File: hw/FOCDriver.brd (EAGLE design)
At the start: 99.1 x 68 mm, 106 parts, among them U1 IX4428N, U2 IX4428N, U3 IX4428N, U4 IRF9389TRPBF, U5 IRF9389TRPBF, U6 IRF9389TRPBF, U7 LM27313XMF, U8 MCP6024T-I, U9 TLV3201AIDBVR

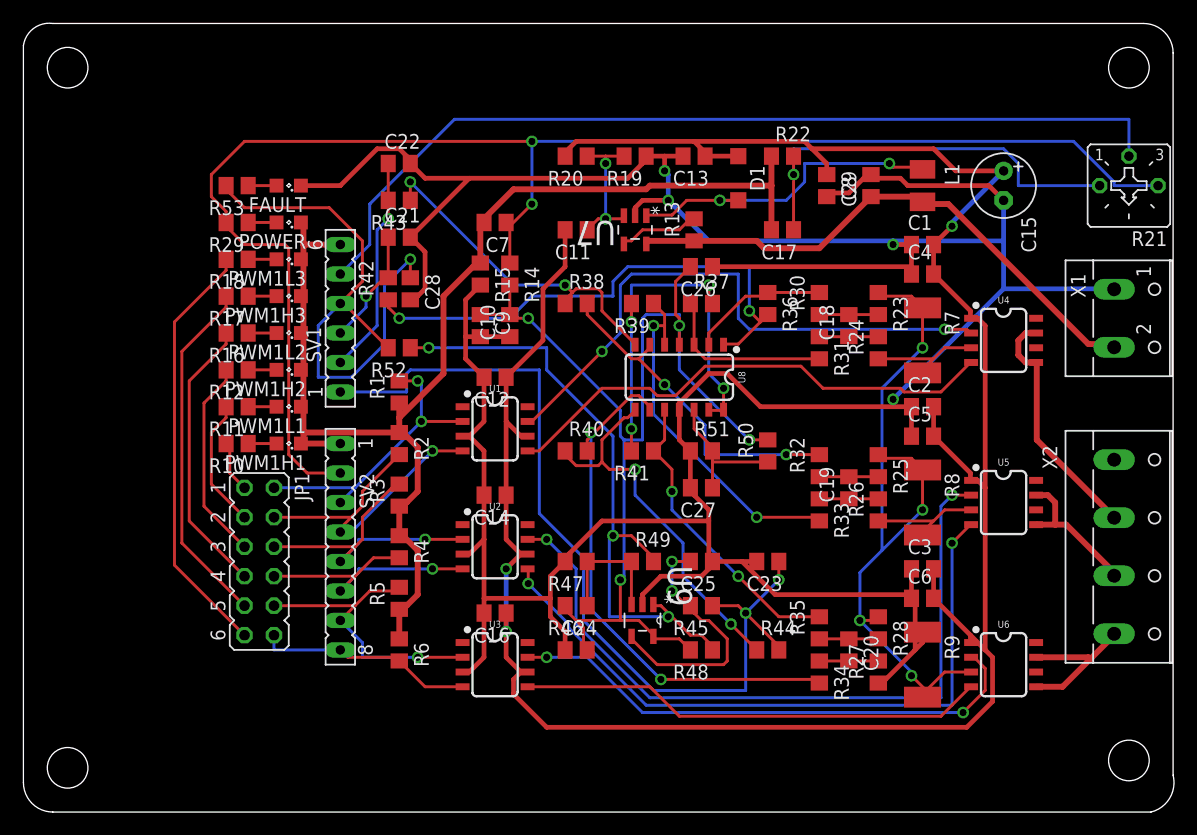
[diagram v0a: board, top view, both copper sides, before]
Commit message: layout
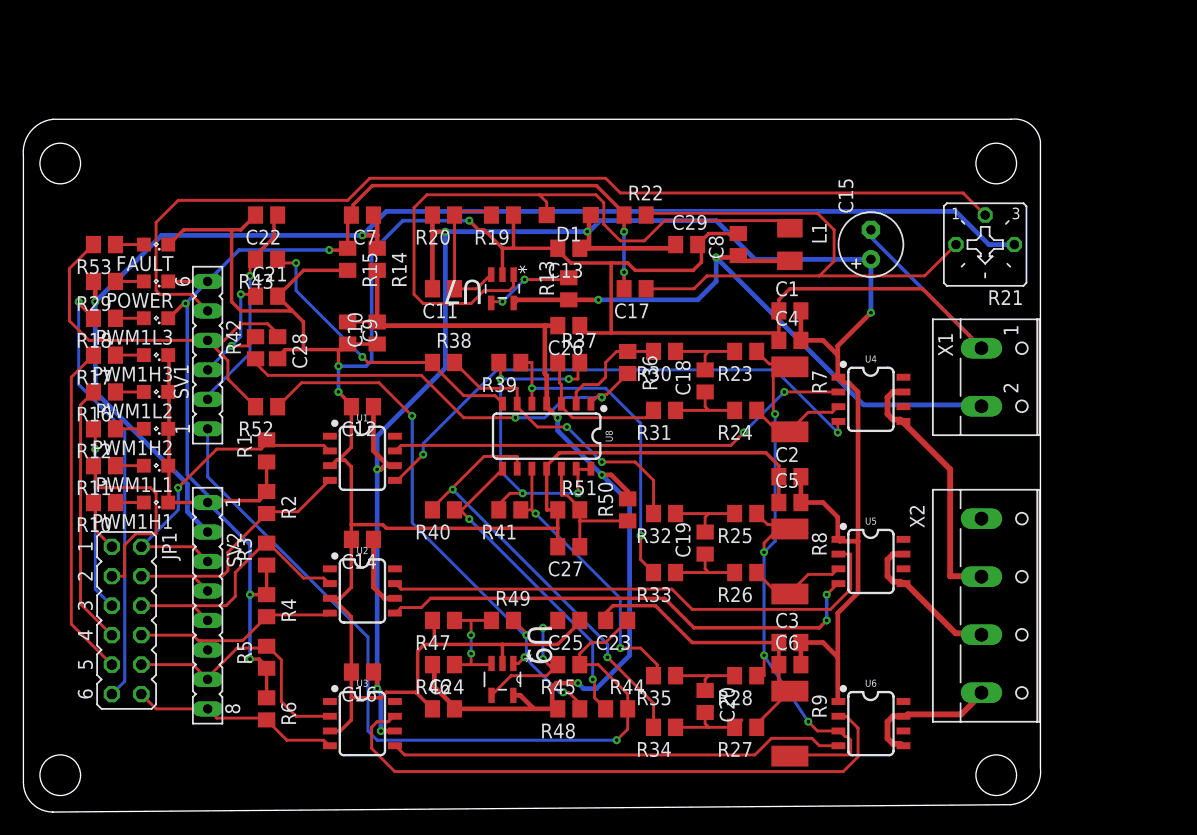
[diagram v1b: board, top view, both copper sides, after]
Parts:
- moved D1 14.9 mm to (47.0, 51.4), turned to 180 degrees
- moved R31 14.4 mm to (55.2, 34.6), turned to 180 degrees
- moved R33 14.4 mm to (55.2, 20.6), turned to 180 degrees
- moved R34 14.2 mm to (55.2, 7.30), turned to 180 degrees
- moved C23 14.0 mm to (51.1, 16.5)
- moved R44 14.0 mm to (51.1, 8.89)
- moved R30 14.0 mm to (55.2, 39.7), turned to 180 degrees
- moved R32 14.0 mm to (55.2, 25.7), turned to 180 degrees
- moved R35 14.0 mm to (55.2, 11.7), turned to 180 degrees
- moved C17 13.7 mm to (52.7, 45.1)
- moved R22 13.7 mm to (52.7, 51.4)
- moved C13 13.4 mm to (47.0, 48.6)
- moved R21 13.4 mm to (82.9, 48.9)
- moved C19 13.3 mm to (58.7, 23.2)
- moved C18 13.3 mm to (58.7, 37.1)
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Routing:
- net N$5: track 28.5 -> 56.6 mm, vias 2 -> 0
- net +12V: track 210.5 -> 183.3 mm, vias 3 -> 6
- net N$8: track 63.6 -> 45.0 mm, vias 2 -> 0
- net +3V3: track 130.9 -> 113.8 mm
- net N$7: track 58.6 -> 42.7 mm
- net FAULT_MC: track 49.8 -> 35.2 mm, vias 1 -> 0
- net N$29: track 37.4 -> 49.6 mm, vias 1 -> 0
- net N$27: track 23.7 -> 12.7 mm
- net N$10: track 50.2 -> 40.3 mm
- net IMOTORBUS: track 78.5 -> 69.3 mm, vias 2 -> 1
- net N$16: track 46.1 -> 37.5 mm
- net AGND: track 314.6 -> 306.0 mm, vias 4 -> 3
- net GND: track 114.8 -> 123.3 mm, vias 0 -> 6
- net N$24: track 46.6 -> 38.2 mm
- net N$1: track 48.4 -> 55.2 mm, vias 0 -> 2
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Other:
- board size 99.1 x 68 mm -> 87.7 x 59.7 mm
